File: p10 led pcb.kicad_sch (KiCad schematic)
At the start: 0 parts

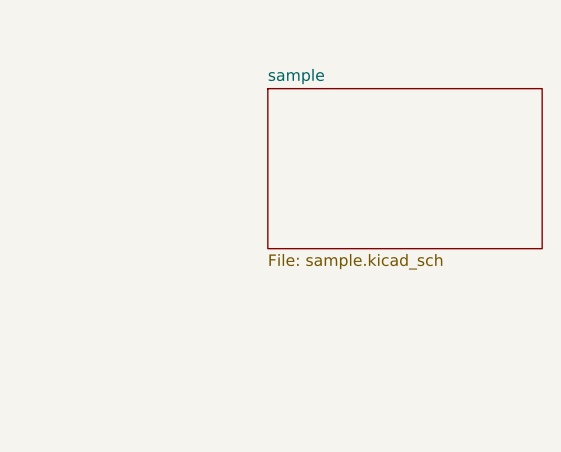
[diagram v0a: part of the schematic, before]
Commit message: Updated PCB
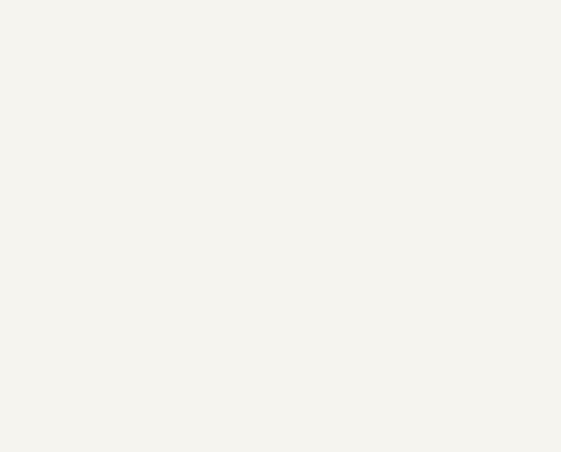
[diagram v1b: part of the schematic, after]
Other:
- removed sheet sample
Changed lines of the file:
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@@
-	)
-	(sheet
-		(at 199.39 43.18)
-		(size 30.48 17.78)
-		(exclude_from_sim no)
-		(in_bom yes)
-		(on_board yes)
-		(dnp no)
-		(fields_autoplaced yes)
-		(stroke
-			(width 0.1524)
-			(type solid)
-		)
-		(fill
-			(color 0 0 0 0)
-		)
-		(property "Sheetname" "sample"
-			(at 199.39 42.4684 0)
-			(show_name no)
-			(do_not_autoplace no)
-			(effects
-				(font
-					(size 1.27 1.27)
-				)
-				(justify left bottom)
-			)
-		)
-		(property "Sheetfile" "sample.kicad_sch"
-			(at 199.39 61.5446 0)
-			(show_name no)
-			(do_not_autoplace no)
-			(effects
-				(font
-					(size 1.27 1.27)
-				)
-				(justify left top)
-			)
-		)
-		(instances
-			(project "p10 led pcb"
-				(path "/eadb67d5-a433-424d-9bb3-9933fead6c55"
-					(page "12")
-				)
-			)
-		)
 	)
 	(sheet

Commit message: sample
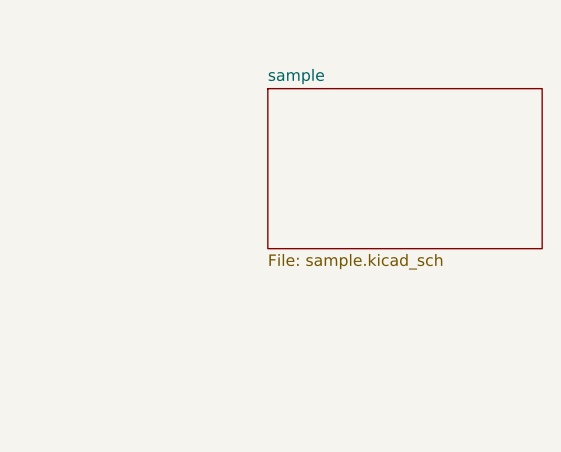
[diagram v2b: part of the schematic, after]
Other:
- added sheet sample (sample.kicad_sch)
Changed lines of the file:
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@@
+	)
+	(sheet
+		(at 199.39 43.18)
+		(size 30.48 17.78)
+		(exclude_from_sim no)
+		(in_bom yes)
+		(on_board yes)
+		(dnp no)
+		(fields_autoplaced yes)
+		(stroke
+			(width 0.1524)
+			(type solid)
+		)
+		(fill
+			(color 0 0 0 0)
+		)
+		(property "Sheetname" "sample"
+			(at 199.39 42.4684 0)
+			(show_name no)
+			(do_not_autoplace no)
+			(effects
+				(font
+					(size 1.27 1.27)
+				)
+				(justify left bottom)
+			)
+		)
+		(property "Sheetfile" "sample.kicad_sch"
+			(at 199.39 61.5446 0)
+			(show_name no)
+			(do_not_autoplace no)
+			(effects
+				(font
+					(size 1.27 1.27)
+				)
+				(justify left top)
+			)
+		)
+		(instances
+			(project "p10 led pcb"
+				(path "/eadb67d5-a433-424d-9bb3-9933fead6c55"
+					(page "12")
+				)
+			)
+		)
 	)
 	(sheet
